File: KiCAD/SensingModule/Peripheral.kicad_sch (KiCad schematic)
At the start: 6 parts, among them J3 TERMISTOR, U10 BME280, U9 BNO055

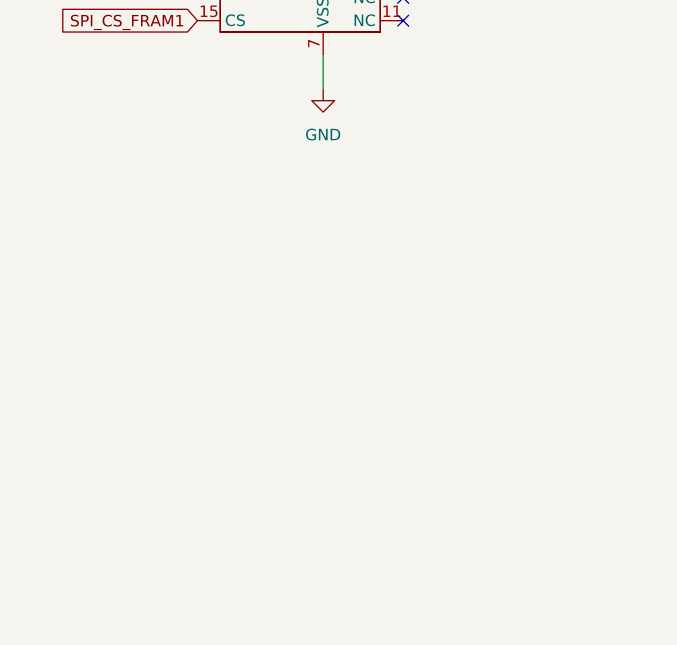
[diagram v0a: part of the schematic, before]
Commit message: 配線確認お願いします
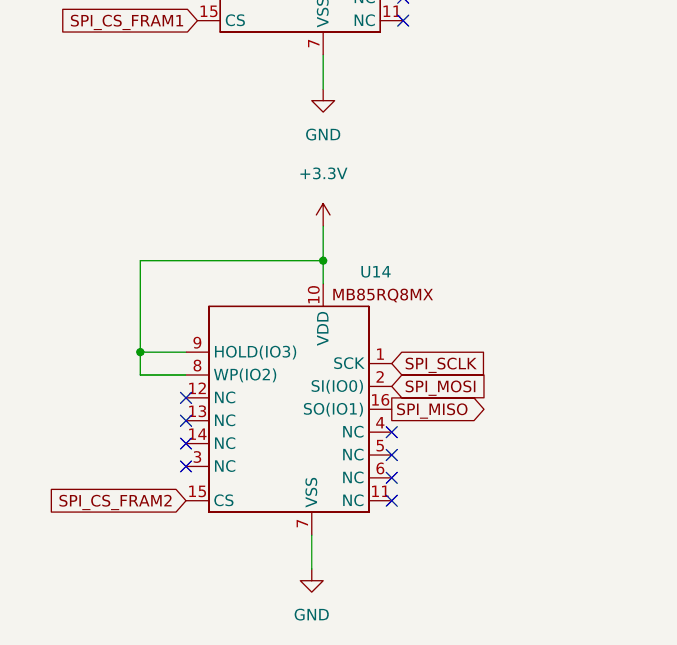
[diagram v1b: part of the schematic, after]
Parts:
- added U14: ~, Package_SO:SOIC-16W_7.5x10.3mm_P1.27mm, symbol MB85RQ8MX_sym:MB85RQMX
- U12, U13: footprint MB85RQ8MX:MB85RQ8MX -> Package_SO:SOIC-16W_7.5x10.3mm_P1.27mm
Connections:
- net +3.3V: now also U14.10 (VDD), U14.8 (WP(IO2)), U14.9 (HOLD(IO3))
- net GND: now also U14.7 (VSS)
- net SPI_MISO: now also U14.16 (SO(IO1))
- net SPI_MOSI: now also U14.2 (SI(IO0))
- net SPI_SCLK: now also U14.1 (SCK)
- new net SPI_CS_FRAM2: U14.15 (CS)
- no-connect marks 19 -> 27
